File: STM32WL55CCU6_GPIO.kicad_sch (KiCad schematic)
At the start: 15 parts, among them IC1 STM32WL55CCU6, J3 BOOT_JPR

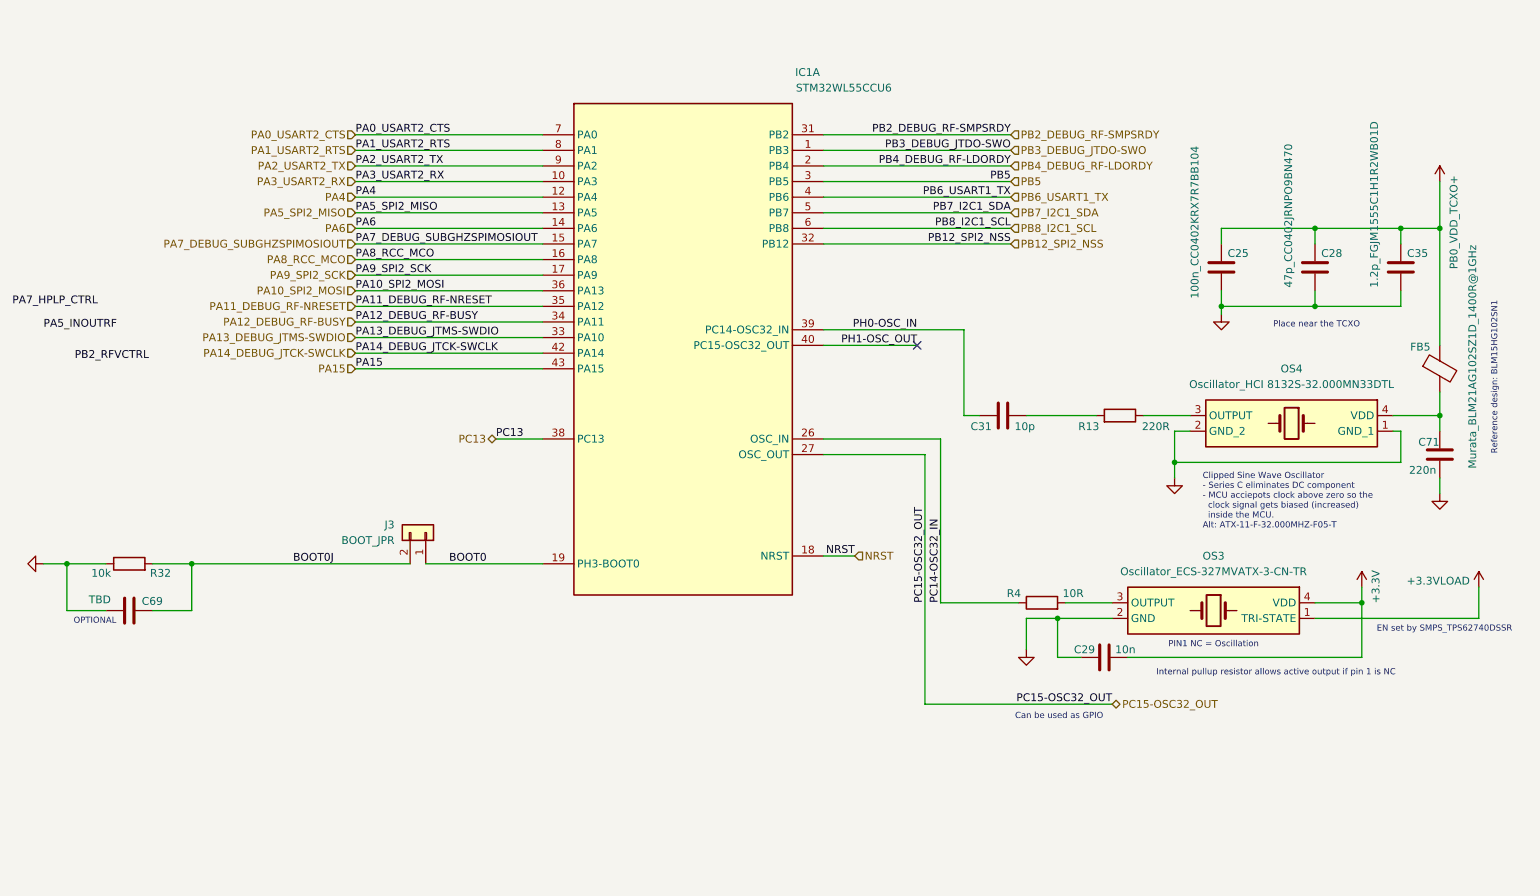
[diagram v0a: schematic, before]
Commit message: PCB Layout
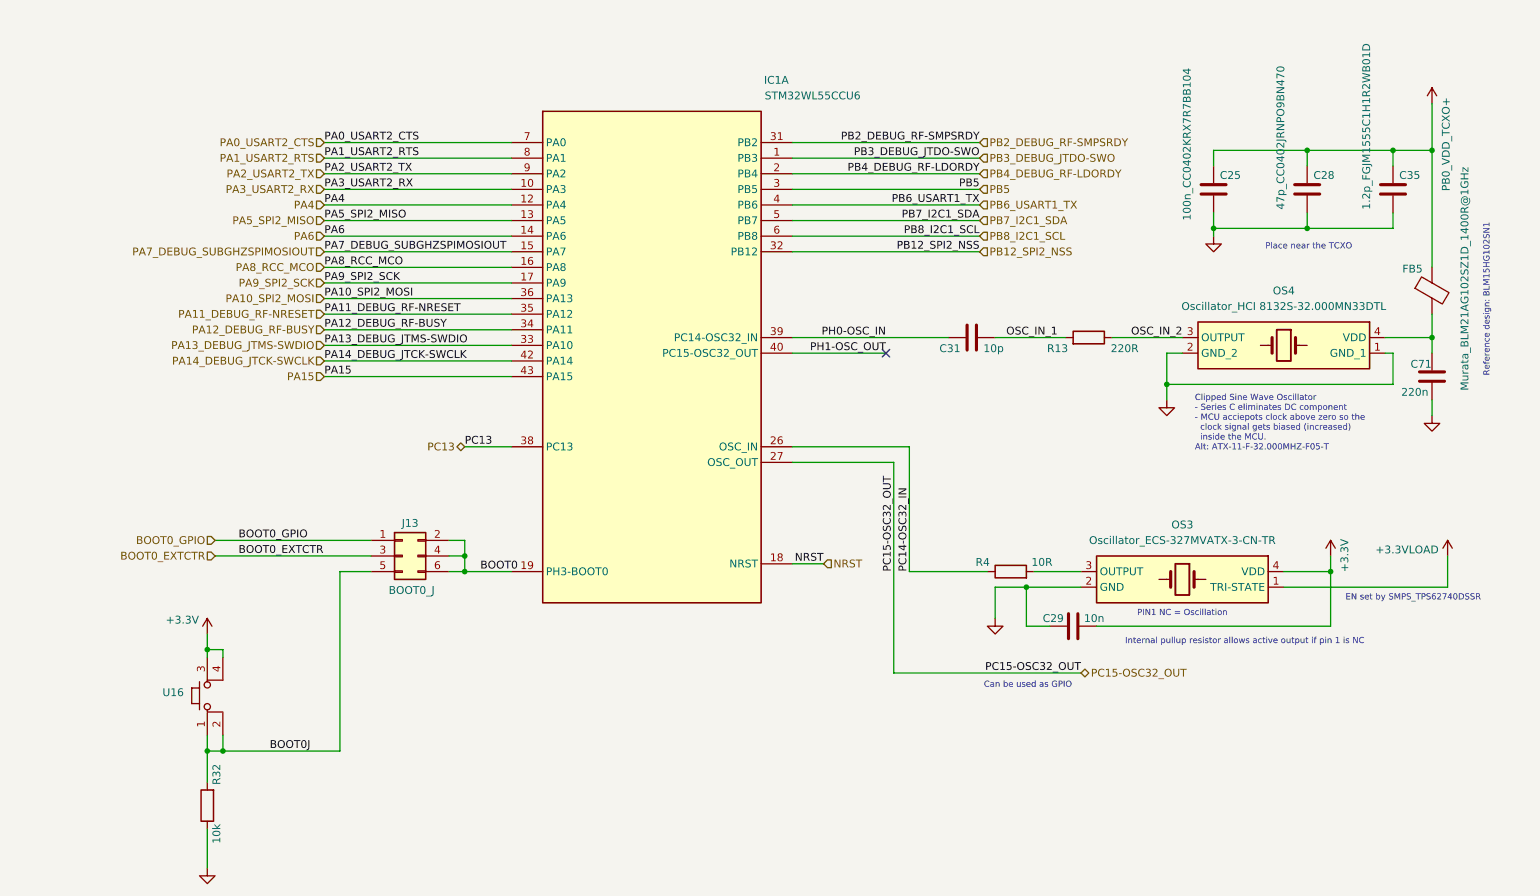
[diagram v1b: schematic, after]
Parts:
- removed C69: TBD, Capacitor_SMD:C_0805_2012Metric, symbol Device:C
- removed J3: BOOT_JPR, symbol Connector_Generic:Conn_01x02
- added J13: BOOT0_J, symbol Connector_Generic:Conn_02x03_Odd_Even
- added U16: (no value), Personal_Project:Button_SKSCLCE010, symbol Personal_Projects:BTN_SKSCLCE010
- C25, C28, C29, C31, C35, C71: footprint Capacitor_SMD:C_0805_2012Metric -> Capacitor_SMD:C_0603_1608Metric
- OS3: footprint Personal_Project:Oscillator_ECS327MVATX3CNTR -> Crystal:Crystal_SMD_3225-4Pin_3.2x2.5mm
- OS4: footprint Personal_Project:Oscillator_ECSTXO32CSMV320ANTR -> Crystal:Crystal_SMD_3225-4Pin_3.2x2.5mm
- R13, R4: footprint Resistor_SMD:R_0805_2012Metric -> Resistor_SMD:R_0603_1608Metric
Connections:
- net +3.3V: now also U16.3, U16.4
- net BOOT0: now also J13.2 (Pin_2), J13.4 (Pin_4), J13.6 (Pin_6)
- net BOOT0J: now also J13.5 (Pin_5), U16.1, U16.2
- net OSC_IN_1: now reaches C31.1, R13.2
- net OSC_IN_2: now reaches OS4.3 (OUTPUT), R13.1
- new net BOOT0_EXTCTR: J13.3 (Pin_3)
- new net BOOT0_GPIO: J13.1 (Pin_1)
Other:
- note removed: "OPTIONAL"
- moved on the sheet: C25, C28, C29, C31, C35, C71, FB5, IC1A, OS3, OS4, R13, R32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
